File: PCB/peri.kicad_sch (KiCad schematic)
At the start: 4 parts, among them J1 Micro_SD_Card, J6 SPI Debug, U4 RN42

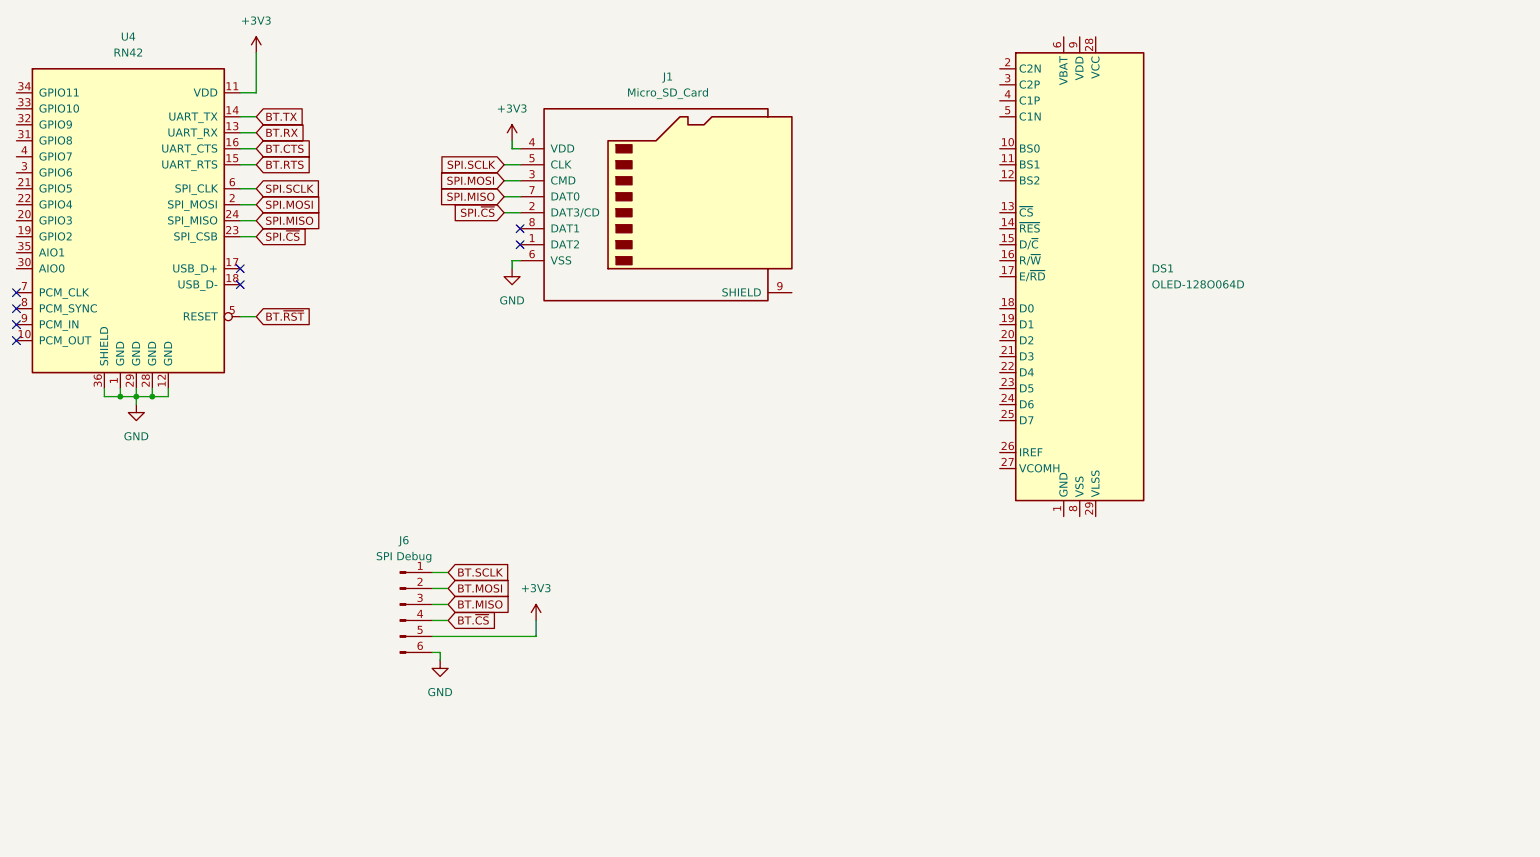
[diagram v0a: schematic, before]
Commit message: PCB update - Minh
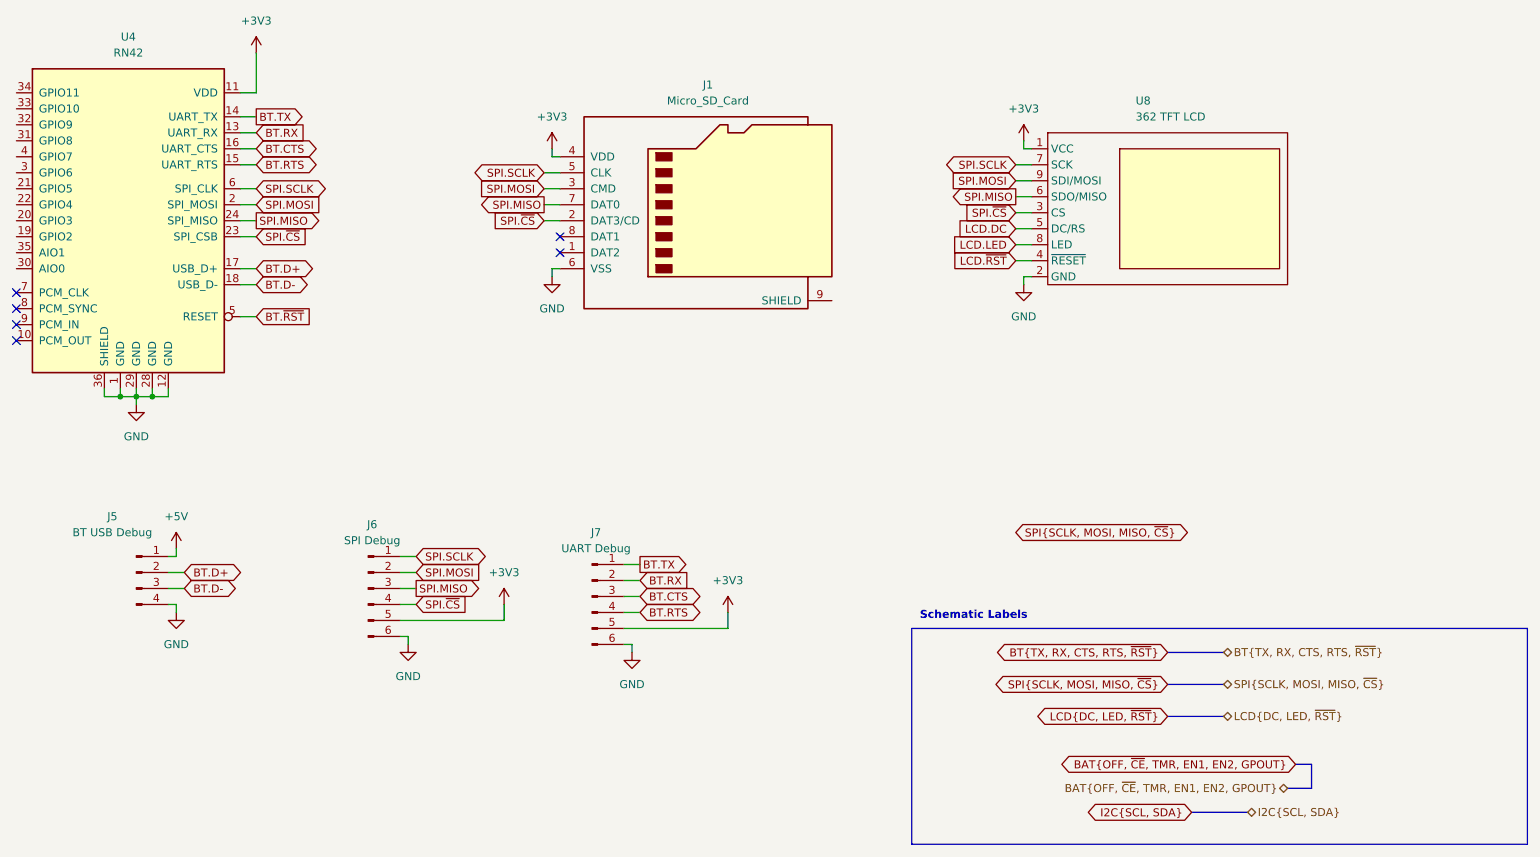
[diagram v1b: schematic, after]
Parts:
- removed DS1: OLED-128O064D, Display:OLED-128O064D, symbol Display_Graphic:OLED-128O064D
- added J5: BT USB Debug, symbol Connector:Conn_01x04_Pin
- added J7: UART Debug, symbol Connector:Conn_01x06_Pin
- added U8: 362 TFT LCD, symbol ECE477_PartsLibrary:362_OLED
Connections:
- net BT.MISO is gone; now on net SPI.MISO: J6.3 (Pin_3)
- net BT.MOSI is gone; now on net SPI.MOSI: J6.2 (Pin_2)
- net BT.SCLK is gone; now on net SPI.SCLK: J6.1 (Pin_1)
- net BT.~{CS} is gone; now on net SPI.~{CS}: J6.4 (Pin_4)
- net +3V3: now also J7.5 (Pin_5), U8.1 (VCC)
- net BT.CTS: now also J7.3 (Pin_3)
- net BT.RTS: now also J7.4 (Pin_4)
- net BT.RX: now also J7.2 (Pin_2)
- net BT.TX: now also J7.1 (Pin_1)
- net GND: now also J5.4 (Pin_4), J7.6 (Pin_6), U8.2 (GND)
- net SPI.MISO: now also U8.6 (SDO/MISO)
- net SPI.MOSI: now also U8.9 (SDI/MOSI)
- net SPI.SCLK: now also U8.7 (SCK)
- net SPI.~{CS}: now also U8.3 (CS)
- net BT.D+: now reaches U4.17 (USB_D+)
- net BT.D+: now also J5.2 (Pin_2)
- net BT.D-: now reaches U4.18 (USB_D-)
- net BT.D-: now also J5.3 (Pin_3)
- new net +5V: J5.1 (Pin_1)
- new net LCD.DC: U8.5 (DC/RS)
- new net LCD.LED: U8.8 (LED)
- new net LCD.~{RST}: U8.4 (~{RESET})
- no-connect marks 8 -> 6
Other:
- note added: "Schematic Labels"
- moved on the sheet: J1, J6

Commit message: Revert "PCB update - Minh"
This reverts commit 0608947e49f54a64abc006b190e3b029bac40ad1.
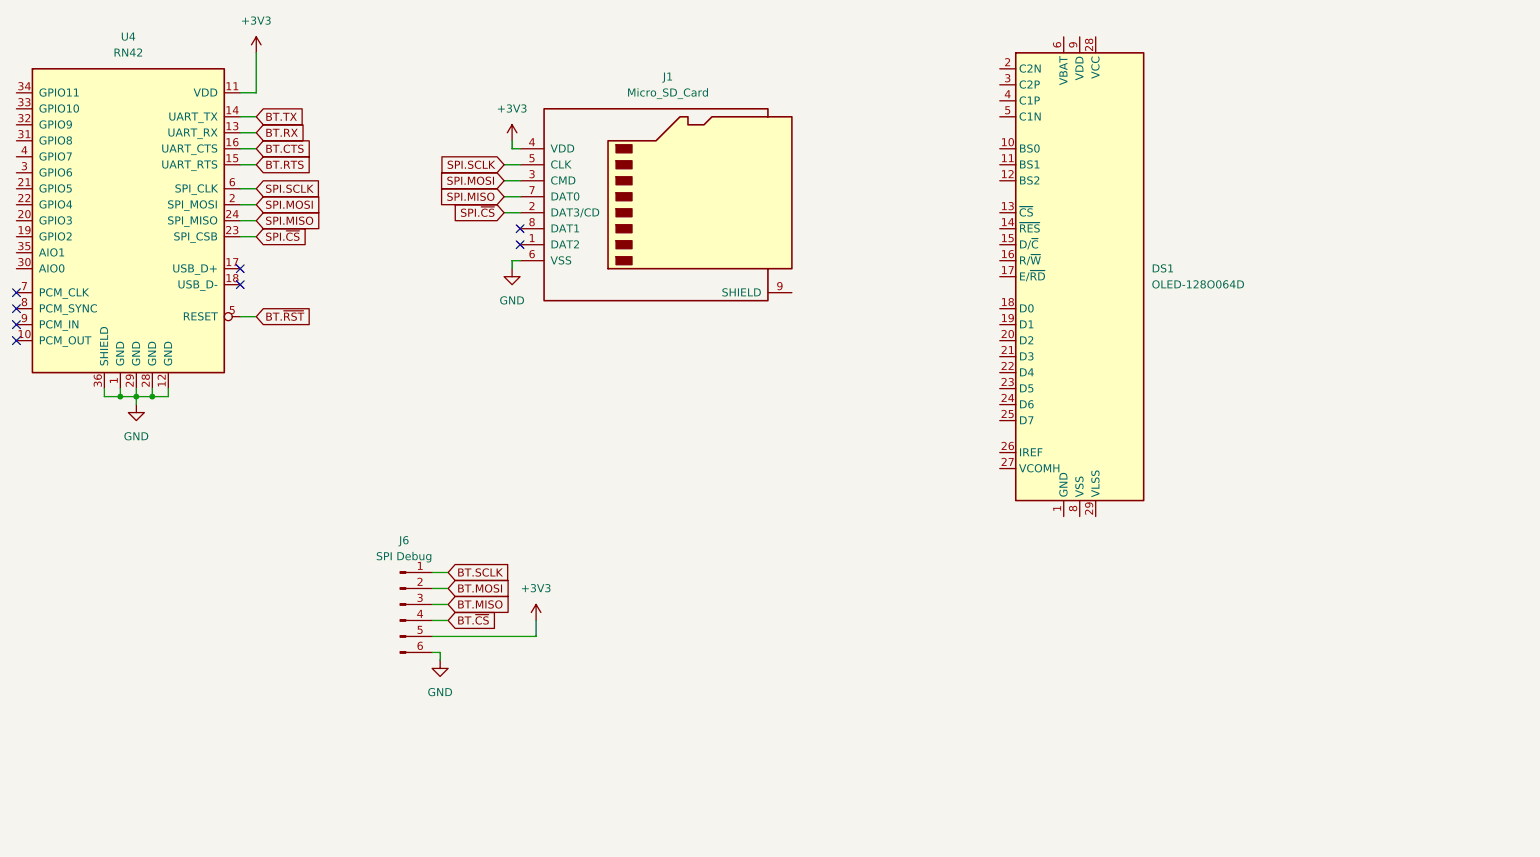
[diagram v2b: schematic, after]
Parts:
- removed J5: BT USB Debug, symbol Connector:Conn_01x04_Pin
- removed J7: UART Debug, symbol Connector:Conn_01x06_Pin
- removed U8: 362 TFT LCD, symbol ECE477_PartsLibrary:362_OLED
- added DS1: OLED-128O064D, Display:OLED-128O064D, symbol Display_Graphic:OLED-128O064D
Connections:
- net SPI.MISO: no longer J6.3 (Pin_3)
- net SPI.MOSI: no longer J6.2 (Pin_2)
- net SPI.SCLK: no longer J6.1 (Pin_1)
- net SPI.~{CS}: no longer J6.4 (Pin_4)
- net BT.D+: no longer names the net of U4.17 (USB_D+)
- net BT.D-: no longer names the net of U4.18 (USB_D-)
- new net: DS1.1 (GND), DS1.30 (GND)
- new net BT.MISO: J6.3 (Pin_3)
- new net BT.MOSI: J6.2 (Pin_2)
- new net BT.SCLK: J6.1 (Pin_1)
- new net BT.~{CS}: J6.4 (Pin_4)
- no-connect marks 6 -> 8
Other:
- note removed: "Schematic Labels"
- moved on the sheet: J1, J6
